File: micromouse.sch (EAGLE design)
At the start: 14 parts

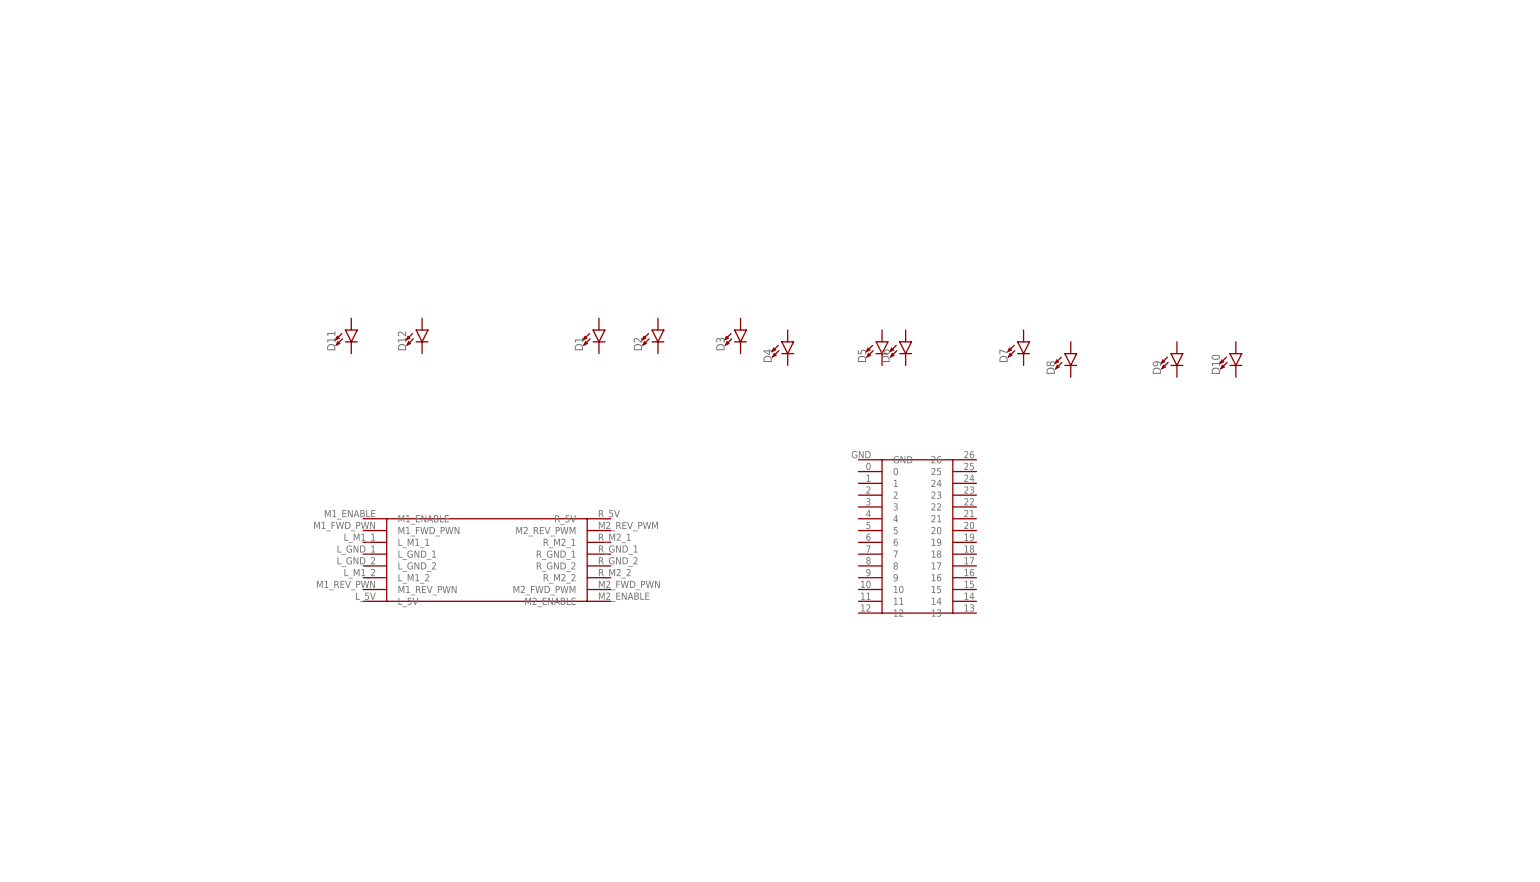
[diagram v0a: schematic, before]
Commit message: Add files via upload
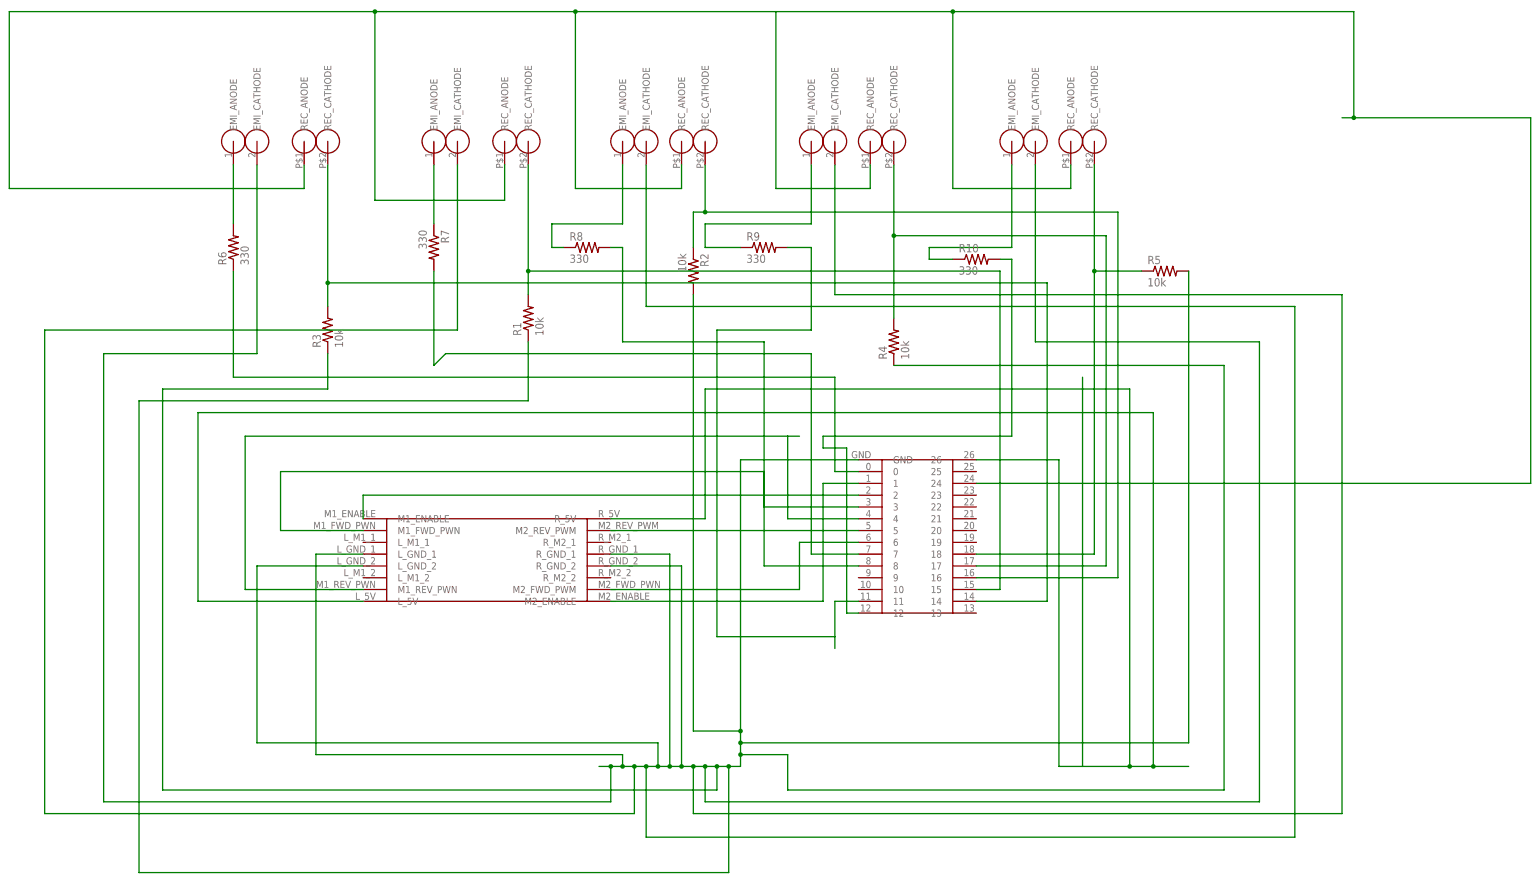
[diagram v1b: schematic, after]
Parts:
- removed D1, D10, D11, D12, D2, D3, D4, D5, D6, D7, D8, D9: (no value), SparkFun_Led:LED5MM-KIT
- added R1, R2, R3, R4, R5: 10k, rcl:R-US_0204/5
- added R10, R6, R7, R8, R9: 330, rcl:R-US_0204/5
- added U$10, U$11, U$12, U$8, U$9: IR_EMITTER, IR_EMITTER:IR_EMITTER
- added U$3, U$4, U$5, U$6, U$7: IR_RECIEVER, IR_RECIEVER:IR_RECIEVER
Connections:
- new net N$1: U$1.2, U$2.M1_ENABLE
- new net N$10: R6.1, U$1.0
- new net N$11: R7.1, U$9.EMI_ANODE
- new net N$12: R7.2, U$1.7
- new net N$13: R8.1, U$10.EMI_ANODE
- new net N$14: R8.2, U$1.8
- new net N$15: R9.1, U$11.EMI_ANODE
- new net N$16: R9.2, U$1.11
- new net N$17: R10.1, U$12.EMI_ANODE
- new net N$18: R10.2, U$1.12
- new net N$19: R1.2, U$1.15, U$4.REC_CATHODE
- new net N$2: U$1.3, U$2.M1_FWD_PWN
- new net N$20: R2.1, U$1.16, U$5.REC_CATHODE
- new net N$21: R4.2, U$1.17, U$6.REC_CATHODE
- new net N$22: R5.1, U$1.18, U$7.REC_CATHODE
- new net N$23: U$1.24, U$3.REC_ANODE, U$4.REC_ANODE, U$5.REC_ANODE, U$6.REC_ANODE, U$7.REC_ANODE
- new net N$24: R3.2, U$1.14, U$3.REC_CATHODE
- new net N$28: R1.1, R2.2, R3.1, R4.1, R5.2, U$1.GND, U$10.EMI_CATHODE, U$11.EMI_CATHODE, U$12.EMI_CATHODE, U$2.L_GND_1, U$2.L_GND_2, U$2.R_GND_1, U$2.R_GND_2, U$8.EMI_CATHODE, U$9.EMI_CATHODE
- new net N$4: U$1.1, U$2.M2_ENABLE
- new net N$5: U$1.5, U$2.M2_REV_PWM
- new net N$6: U$1.26, U$2.L_5V, U$2.R_5V
- new net N$7: U$1.6, U$2.M2_FWD_PWM
- new net N$8: U$1.4, U$2.M1_REV_PWN
- new net N$9: R6.2, U$8.EMI_ANODE
